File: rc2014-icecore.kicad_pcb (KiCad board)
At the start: 2 copper layers, 99.3 x 60.1 mm, 21 parts, among them J1 Conn_01x39, J2 Conn_01x10, J3 Conn_02x15_Odd_Even, J4 Conn_02x13_Odd_Even, U1 LM1117-3.3, U2 SN74CB3T3245, U3 SN74CB3T3245, U4 SN74CB3T3245, U5 SN74CB3T3245, U6 SN74CB3T3245

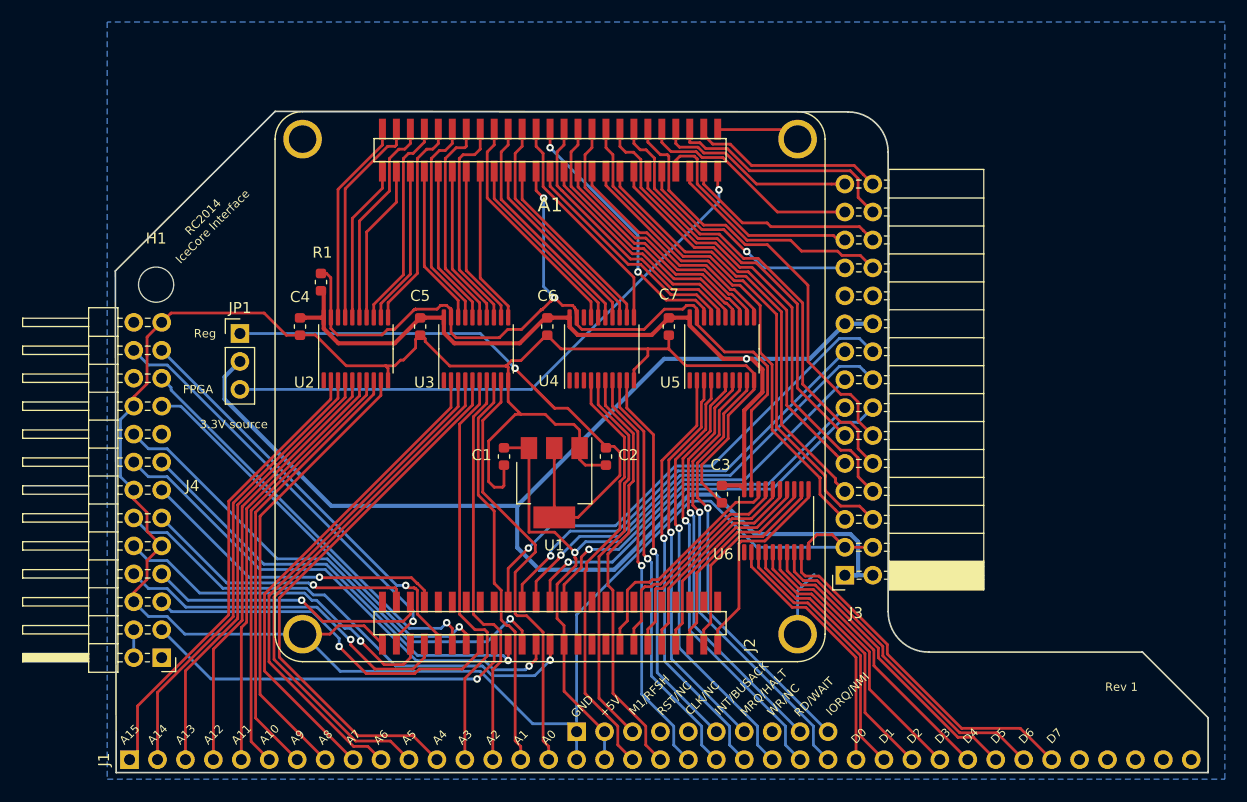
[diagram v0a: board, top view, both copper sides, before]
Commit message: WIP
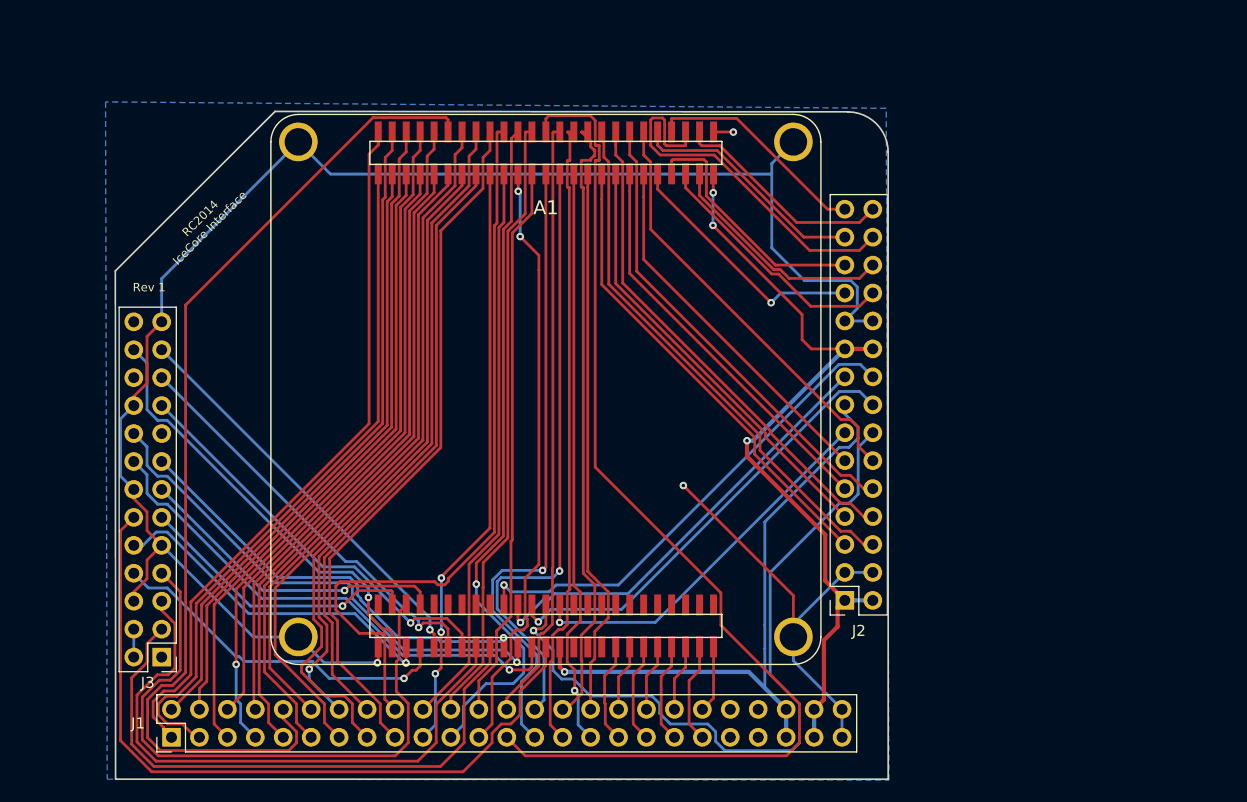
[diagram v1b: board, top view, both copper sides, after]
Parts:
- removed C1: 100nF, Capacitor_SMD:C_0603_1608Metric
- removed C2: 10uF, Capacitor_SMD:C_0603_1608Metric
- removed C3, C4, C5, C6, C7: C, Capacitor_SMD:C_0603_1608Metric
- removed H1: MountingHole, MountingHole:MountingHole_3.2mm_M3
- removed J4: Conn_02x13_Odd_Even, Connector_PinHeader_2.54mm:PinHeader_2x13_P2.54mm_Horizontal
- removed JP1: Ext Power, Connector_PinHeader_2.54mm:PinHeader_1x03_P2.54mm_Vertical
- removed R1: R, Resistor_SMD:R_0603_1608Metric
- removed U1: LM1117-3.3, Package_TO_SOT_SMD:SOT-223-3_TabPin2
- removed U2, U3, U4, U5, U6: SN74CB3T3245, Package_SO:TSSOP-20_4.4x6.5mm_P0.65mm
- J1: value Conn_01x39 -> Conn_02x25_Odd_Even; footprint rc2014:PinHeader_1x39_P2.54mm_Vertical_NoSilk -> Connector_PinHeader_2.54mm:PinHeader_2x25_P2.54mm_Vertical
- J2: value Conn_01x10 -> Conn_02x15_Odd_Even; footprint rc2014:PinHeader_1x10_P2.54mm_Vertical_NoSilk -> Connector_PinSocket_2.54mm:PinSocket_2x15_P2.54mm_Vertical
- J3: value Conn_02x15_Odd_Even -> Conn_02x13_Odd_Even; footprint Connector_PinSocket_2.54mm:PinSocket_2x15_P2.54mm_Horizontal -> Connector_PinHeader_2.54mm:PinHeader_2x13_P2.54mm_Vertical
- moved J3 62.5 mm to (64.6, 154.0)
- moved J2 27.1 mm to (126.7, 148.8), turned to 180 degrees
- moved J1 4.32 mm to (65.5, 161.3)
- moved A1 0.46 mm to (84.3, 106.2)
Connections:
- J1 pad 1: /A15 -> /P0
- J1 pad 10: /A6 -> /P9
- J1 pad 11: /A5 -> /P10
- J1 pad 12: /A4 -> /P11
- J1 pad 13: /A3 -> /P12
- J1 pad 14: /A2 -> /P13
- J1 pad 15: /A1 -> /P14
- J1 pad 16: /A0 -> /P15
- J1 pad 17: GND -> /P16
- J1 pad 18: +5V -> /P17
- J1 pad 19: /M1 -> /P18
- J1 pad 2: /A14 -> /P1
- J1 pad 20: //RESET -> /P19
- J1 pad 21: /CLK -> /P20
- J1 pad 22: /INT -> /P21
- J1 pad 23: /MREQ -> /P22
- J1 pad 24: //WR -> /P23
- J1 pad 25: //RD -> /P24
- J1 pad 26: //IORQ -> /P25
- J1 pad 27: /D0 -> /P26
- J1 pad 28: /D1 -> /P27
- J1 pad 29: /D2 -> /P28
- J1 pad 3: /A13 -> /P2
- J1 pad 30: /D3 -> /P29
- J1 pad 31: /D4 -> /P30
- J1 pad 32: /D5 -> /P31
- J1 pad 33: /D6 -> /P48
- J1 pad 34: /D7 -> /P49
- J1 pad 35: (no net) -> /P50
- J1 pad 36: (no net) -> /P51
- J1 pad 37: (no net) -> /P52
- J1 pad 38: (no net) -> /P53
- J1 pad 39: (no net) -> /P54
- J1 pad 4: /A12 -> /P3
- J1 pad 5: /A11 -> /P4
- J1 pad 6: /A10 -> /P5
- J1 pad 7: /A9 -> /P6
- J1 pad 8: /A8 -> /P7
- J1 pad 9: /A7 -> /P8
- J2 pad 1: GND -> /FPGA_VCC
- J2 pad 10: /~NMI -> /P36
- J2 pad 2: +5V -> /FPGA_VCC
- J2 pad 3: /~RFSH -> GND
- J2 pad 4: (no net) -> GND
- J2 pad 5: (no net) -> /P34
- J2 pad 6: /BUSACK -> /P32
- J2 pad 7: /~HALT -> /P35
- J2 pad 8: (no net) -> /P33
- J2 pad 9: /~WAIT -> /P38
- J3 pad 1: +3V3 -> (no net)
- J3 pad 10: /P36 -> /TX
- J3 pad 11: /P39 -> /SWDIO
- J3 pad 12: /P37 -> /TCK
- J3 pad 13: /AN9 -> /~RESET
- J3 pad 14: /AN8 -> GND
- J3 pad 15: +5V -> /TMS
- J3 pad 16: /AN7 -> /TDI
- J3 pad 17: /AN6 -> (no net)
- J3 pad 18: /AN5 -> /TDO
- J3 pad 19: +3V3 -> /EMOSI
- J3 pad 2: +3V3 -> Net-(J3-Pad2)
- J3 pad 20: +3V3 -> GND
- J3 pad 21: GND -> /EMISO
- J3 pad 22: GND -> (no net)
- J3 pad 23: /P42 -> /ESCK
- J3 pad 24: /P46 -> /~ESS
- J3 pad 25: /P43 -> GND
- J3 pad 26: /P47 -> (no net)
- J3 pad 3: GND -> /SDA
- J3 pad 4: GND -> Net-(J3-Pad2)
- J3 pad 5: /P34 -> /SCL
- J3 pad 6: /P32 -> GND
- J3 pad 7: /P35 -> /SWCLK
- J3 pad 8: /P33 -> /RX
- J3 pad 9: /P38 -> GND
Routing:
- net +3V3: track 188.6 -> 0.00 mm, vias 1 -> 0
- net /P24: track 24.5 -> 98.7 mm, vias 2 -> 0
- net /P9: track 19.5 -> 91.3 mm
- net GND: track 257.3 -> 187.6 mm, vias 0 -> 3
- net Net-(C2-Pad1): track 57.8 -> 0.00 mm, vias 1 -> 0
- net /A4: track 50.6 -> 0.00 mm
- net /A5: track 48.6 -> 0.00 mm
- net /P2: track 14.4 -> 62.6 mm
- net /P17: track 21.3 -> 68.7 mm
- net /P14: track 14.6 -> 61.4 mm
- net /A6: track 46.6 -> 0.00 mm
- net /P0: track 18.8 -> 64.8 mm
- net /A7: track 44.8 -> 0.00 mm
- net /P12: track 19.7 -> 64.5 mm
- net /P10: track 14.6 -> 59.4 mm
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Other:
- board size 99.3 x 60.1 mm -> 70.3 x 60.7 mm
- board text added: "github.com/electrified/rc2014-icecore"
- board text removed: "+5V"
- board text removed: "3.3V source"
- board text removed: "A0"
- board text removed: "A1"
- board text removed: "A10"
- board text removed: "A11"
- board text removed: "A12"
- board text removed: "A13"
- board text removed: "A14"
- board text removed: "A15"
- board text removed: "A2"
- board text removed: "A3"
- board text removed: "A4"
- board text removed: "A5"
- board text removed: "A6"
- board text removed: "A7"
- board text removed: "A8"
- board text removed: "A9"
- board text removed: "CLK/NC"
- board text removed: "D0"
- board text removed: "D1"
- board text removed: "D2"
- board text removed: "D3"
- board text removed: "D4"
- board text removed: "D5"
- board text removed: "D6"
- board text removed: "D7"
- board text removed: "FPGA"
- board text removed: "GND"
- board text removed: "INT/BUSACK"
- board text removed: "IORQ/NMI"
- board text removed: "M1/RFSH"
- board text removed: "MRQ/HALT"
- board text removed: "RD/WAIT"
- board text removed: "RST/NC"
- board text removed: "Reg"
- board text removed: "WR/NC"
- board text removed: "github.com/electrified/rc2014-fpga-interface"
